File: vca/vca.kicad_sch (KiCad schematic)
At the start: 20 parts, among them U4 STM32F103C6Tx, Y1 Crystal_8Mhz

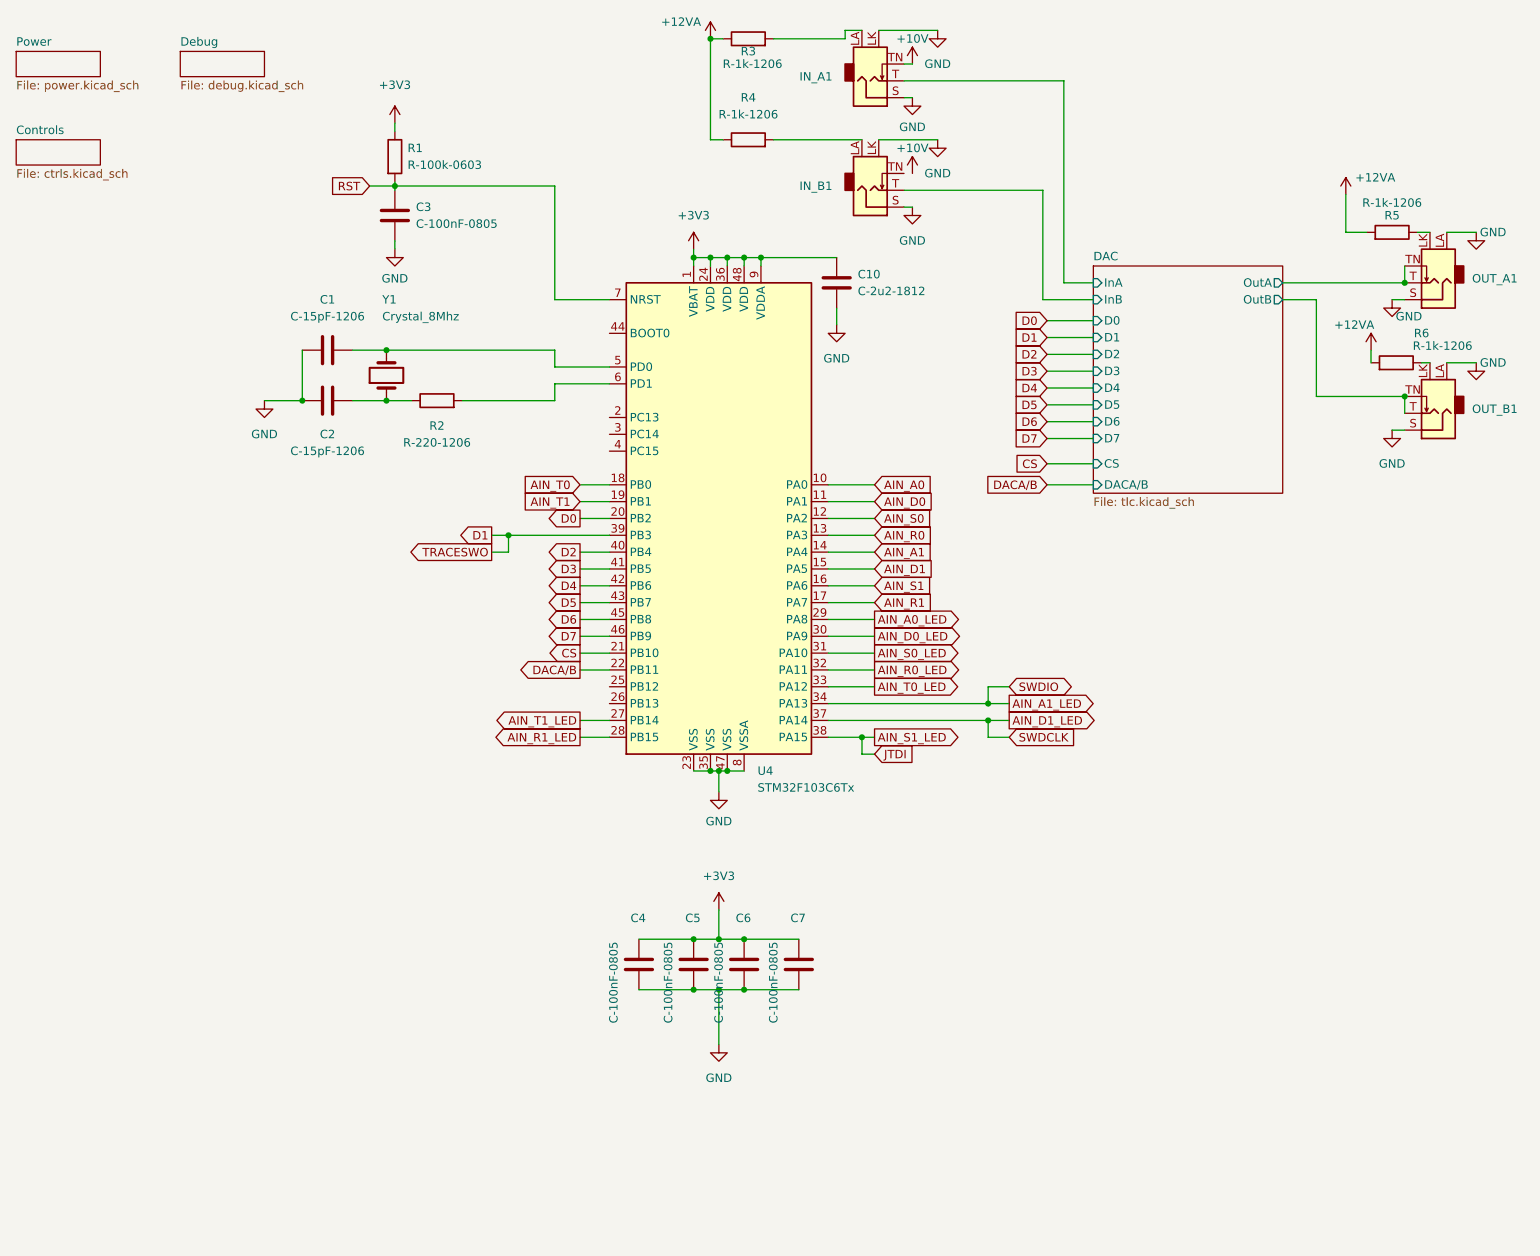
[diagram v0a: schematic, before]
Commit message: working on the PCB
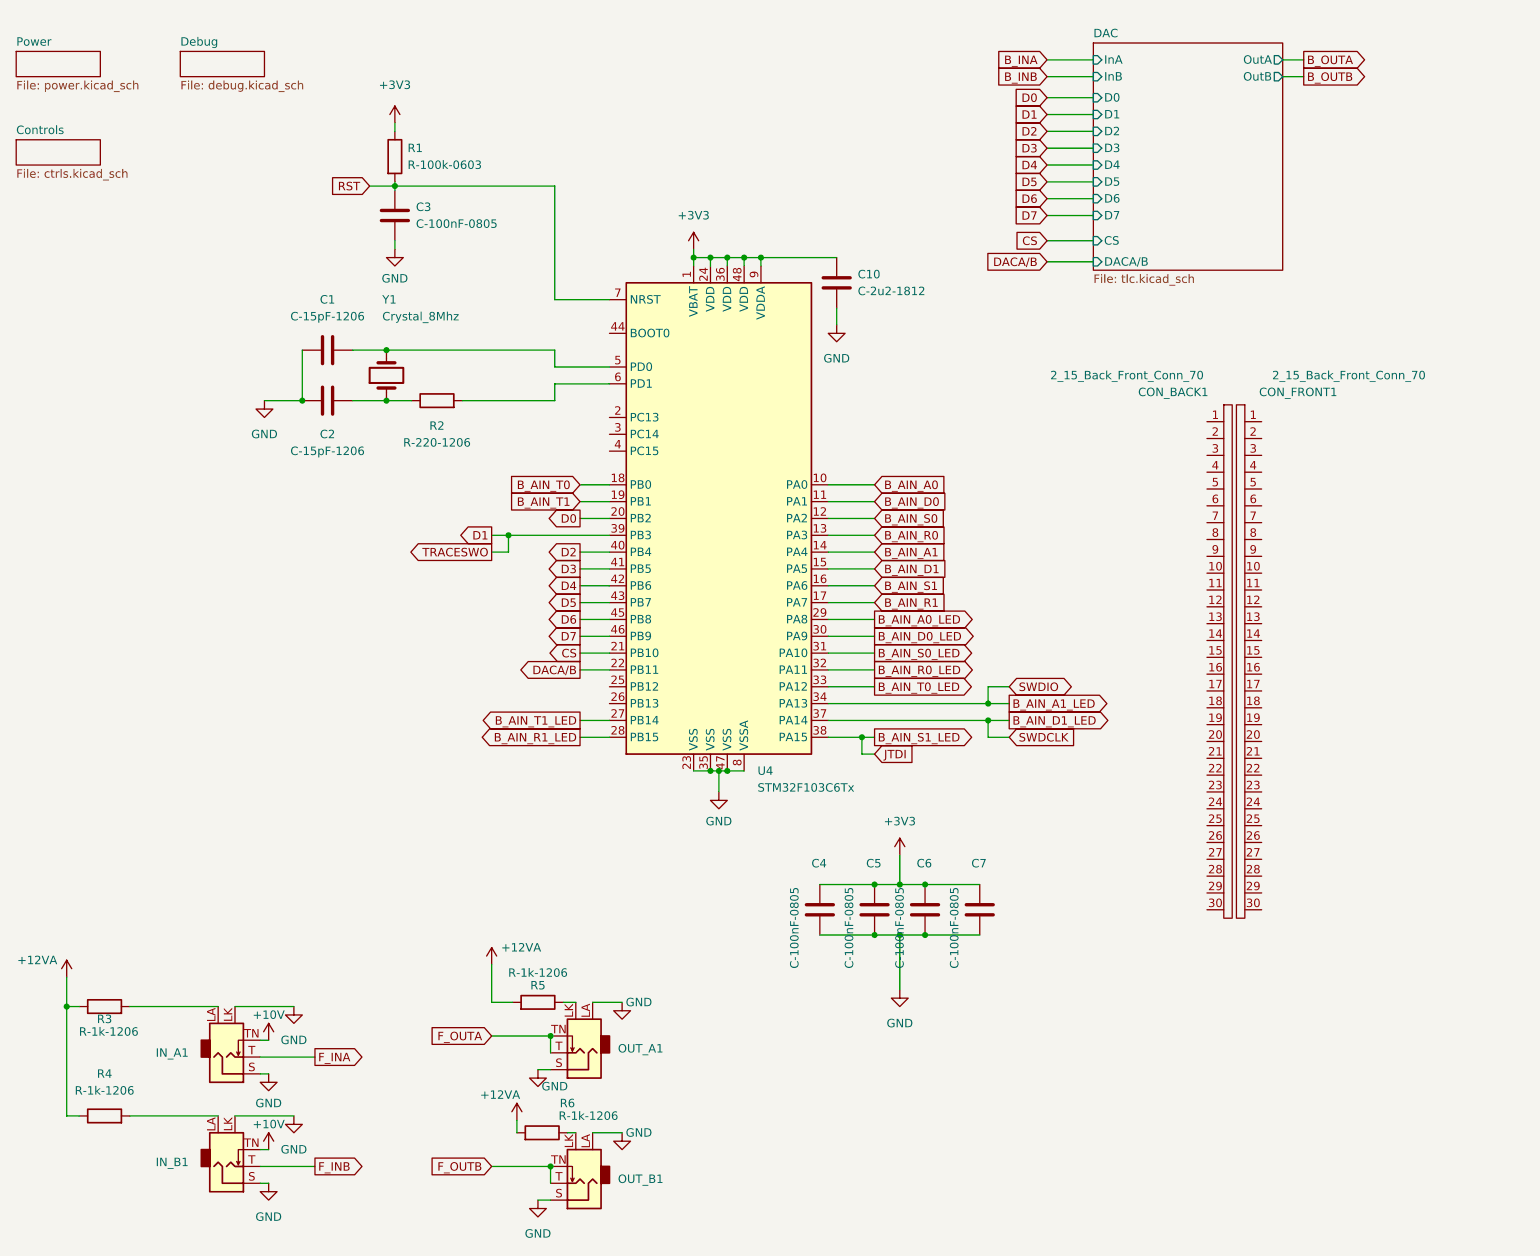
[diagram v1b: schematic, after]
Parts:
- added CON_BACK1, CON_FRONT1: 2_15_Back_Front_Conn_70, eurorack:2_15_back_front_conn_70, symbol eurorack:2_15_Back_Front_Conn_70
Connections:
- net +10V: now also IN_B1.TN
- net AIN_A0 renamed B_AIN_A0
- net AIN_A0_LED renamed B_AIN_A0_LED
- net AIN_A1 renamed B_AIN_A1
- net AIN_A1_LED renamed B_AIN_A1_LED
- net AIN_D0 renamed B_AIN_D0
- net AIN_D0_LED renamed B_AIN_D0_LED
- net AIN_D1 renamed B_AIN_D1
- net AIN_D1_LED renamed B_AIN_D1_LED
- net AIN_R0 renamed B_AIN_R0
- net AIN_R0_LED renamed B_AIN_R0_LED
- net AIN_R1 renamed B_AIN_R1
- net AIN_R1_LED renamed B_AIN_R1_LED
- net AIN_S0 renamed B_AIN_S0
- net AIN_S0_LED renamed B_AIN_S0_LED
- net AIN_S1 renamed B_AIN_S1
- net AIN_S1_LED renamed B_AIN_S1_LED
- net AIN_T0 renamed B_AIN_T0
- net AIN_T0_LED renamed B_AIN_T0_LED
- net AIN_T1 renamed B_AIN_T1
- net AIN_T1_LED renamed B_AIN_T1_LED
- net DAC/InA renamed F_INA
- net DAC/InB renamed F_INB
- net DAC/OutA renamed F_OUTA
- net DAC/OutB renamed F_OUTB
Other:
- moved on the sheet: C4, C5, C6, C7, IN_A1, IN_B1, OUT_A1, OUT_B1, R3, R4, R5, R6

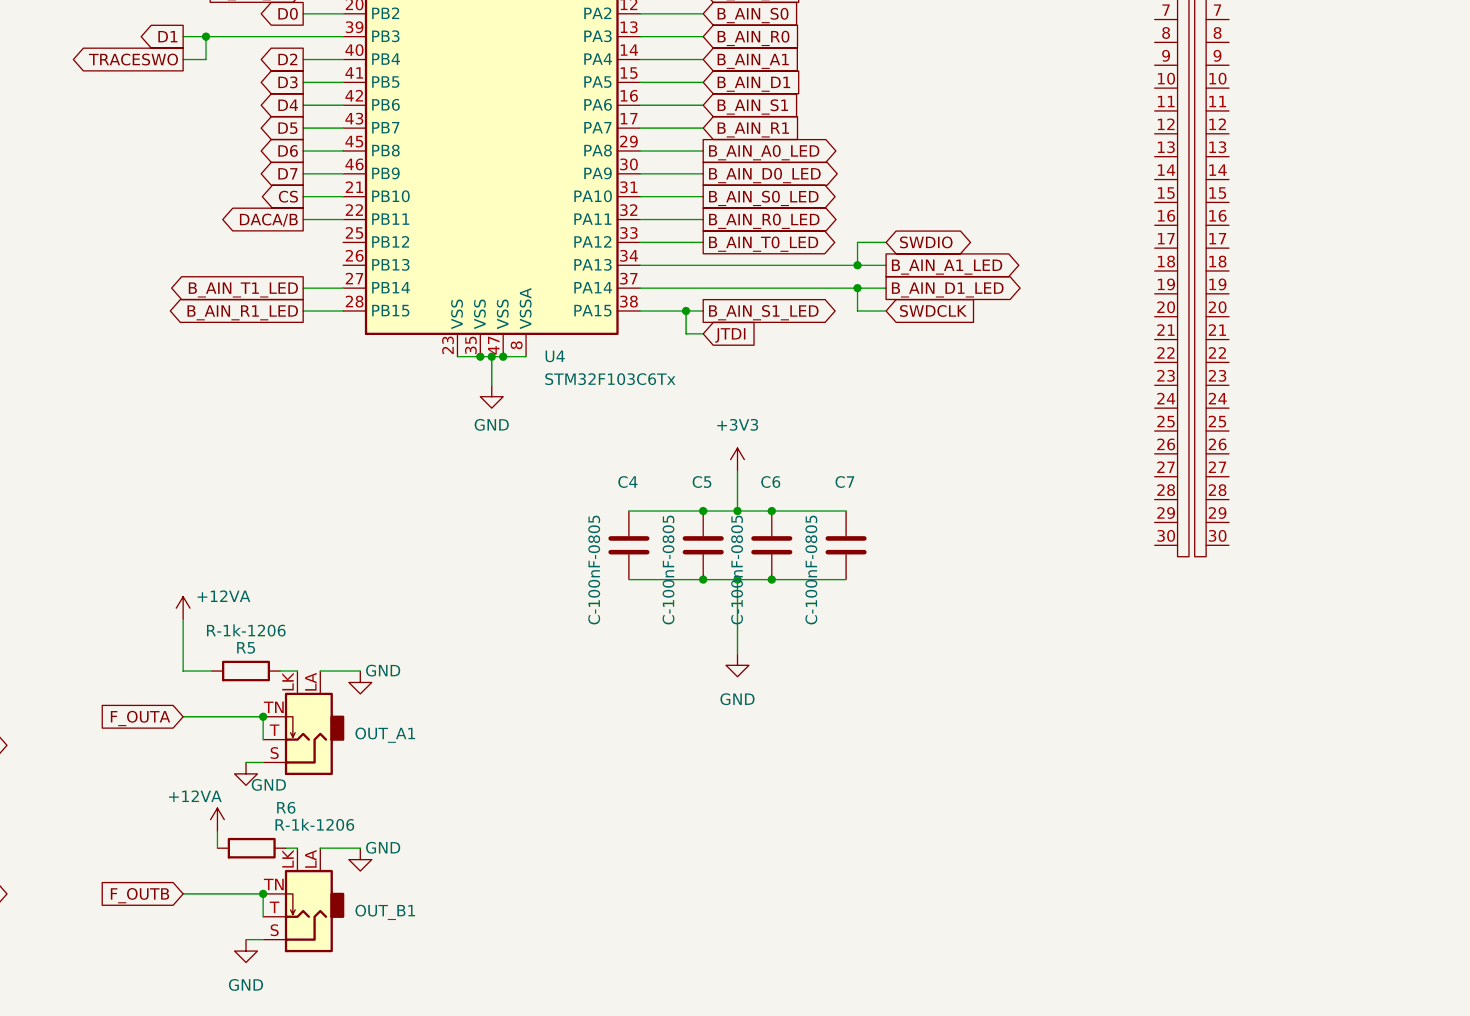
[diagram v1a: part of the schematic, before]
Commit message: working on front panel
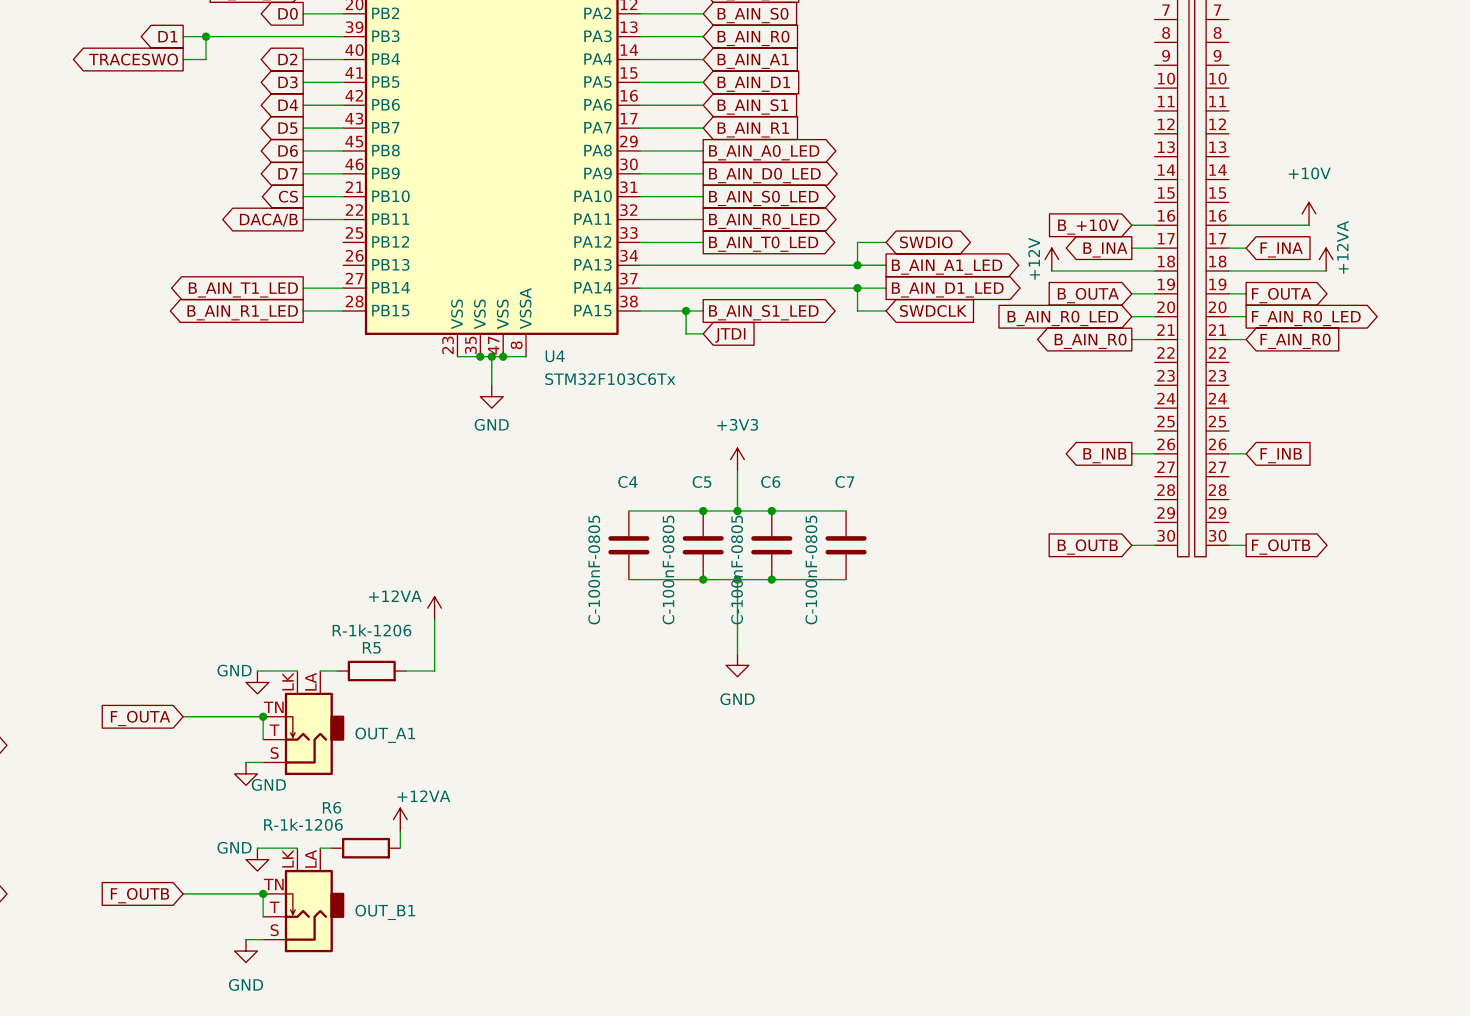
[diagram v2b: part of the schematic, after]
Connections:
- net +10V: now also CON_FRONT1.16
- net +12VA: now also CON_FRONT1.18
- net B_AIN_R0: now also CON_BACK1.21
- net B_AIN_R0_LED: now also CON_BACK1.20
- net B_INA: now also CON_BACK1.17
- net B_INB: now also CON_BACK1.26
- net B_OUTA: now also CON_BACK1.19
- net B_OUTB: now also CON_BACK1.30
- net F_INA: now also CON_FRONT1.17
- net F_INB: now also CON_FRONT1.26
- net F_OUTA: now also CON_FRONT1.19
- net F_OUTB: now also CON_FRONT1.30
- net GND: now also OUT_A1.LK, OUT_B1.LK; no longer OUT_A1.LA, OUT_B1.LA
- net at R6.1: now also OUT_B1.LA; no longer OUT_B1.LK
- net B_+10V: now reaches CON_BACK1.16
- net +12V: now reaches CON_BACK1.18
- net at R5.1: now also OUT_A1.LA; no longer OUT_A1.LK
- net F_AIN_R0_LED: now reaches CON_FRONT1.20
- net F_AIN_R0: now reaches CON_FRONT1.21
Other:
- moved on the sheet: R5, R6

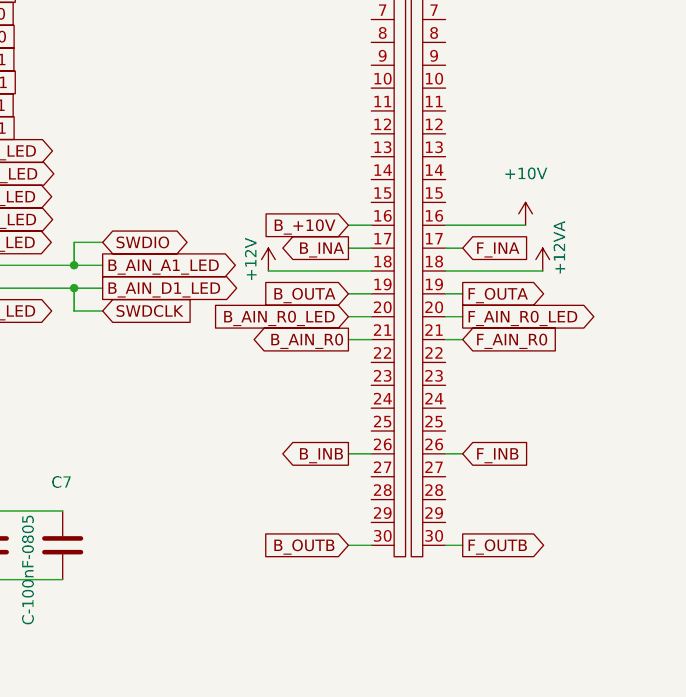
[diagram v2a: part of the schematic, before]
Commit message: working on the front panel
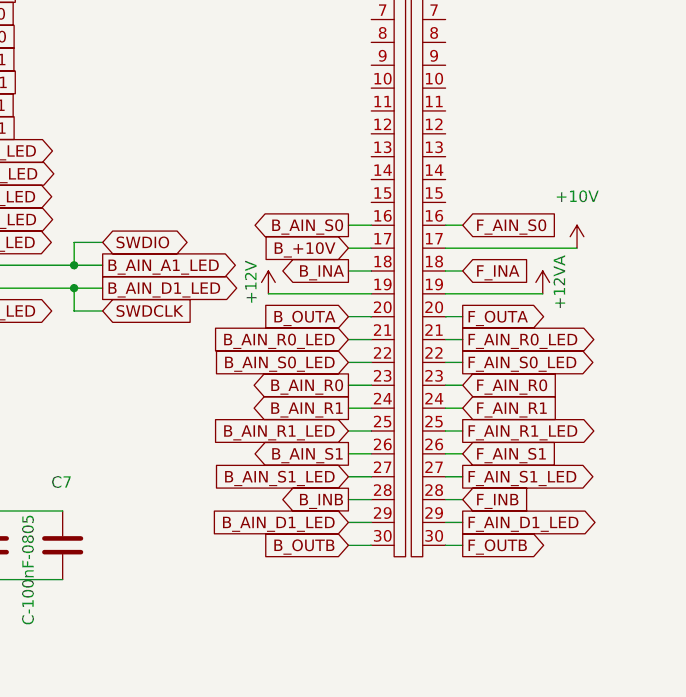
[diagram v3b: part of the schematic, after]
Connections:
- net +10V: now also CON_FRONT1.17; no longer CON_FRONT1.16
- net +12V: now also CON_BACK1.19; no longer CON_BACK1.18
- net +12VA: now also CON_FRONT1.19; no longer CON_FRONT1.18
- net B_+10V: now also CON_BACK1.17; no longer CON_BACK1.16
- net B_AIN_D1_LED: now also CON_BACK1.29
- net B_AIN_R0: now also CON_BACK1.23; no longer CON_BACK1.21
- net B_AIN_R0_LED: now also CON_BACK1.21; no longer CON_BACK1.20
- net B_AIN_R1: now also CON_BACK1.24
- net B_AIN_R1_LED: now also CON_BACK1.25
- net B_AIN_S0: now also CON_BACK1.16
- net B_AIN_S0_LED: now also CON_BACK1.22
- net B_AIN_S1: now also CON_BACK1.26
- net B_AIN_S1_LED: now also CON_BACK1.27
- net B_INA: now also CON_BACK1.18; no longer CON_BACK1.17
- net B_INB: now also CON_BACK1.28; no longer CON_BACK1.26
- net B_OUTA: now also CON_BACK1.20; no longer CON_BACK1.19
- net F_AIN_R0: now also CON_FRONT1.23; no longer CON_FRONT1.21
- net F_AIN_R0_LED: now also CON_FRONT1.21; no longer CON_FRONT1.20
- net F_INA: now also CON_FRONT1.18; no longer CON_FRONT1.17
- net F_INB: now also CON_FRONT1.28; no longer CON_FRONT1.26
- net F_OUTA: now also CON_FRONT1.20; no longer CON_FRONT1.19
- net F_AIN_S0_LED: now reaches CON_FRONT1.22
- net F_AIN_R1: now reaches CON_FRONT1.24
- net F_AIN_R1_LED: now reaches CON_FRONT1.25
- net F_AIN_S1_LED: now reaches CON_FRONT1.27
- net F_AIN_D1_LED: now reaches CON_FRONT1.29
- new net F_AIN_S0: CON_FRONT1.16
- new net F_AIN_S1: CON_FRONT1.26

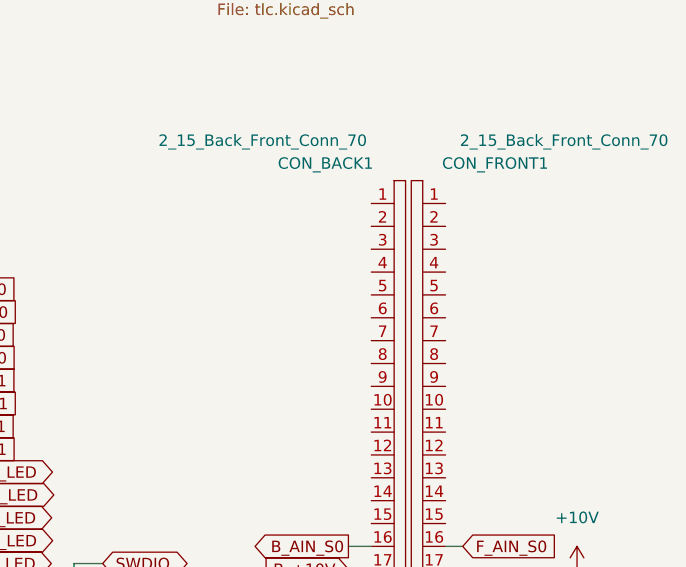
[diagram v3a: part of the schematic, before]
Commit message: working on the front
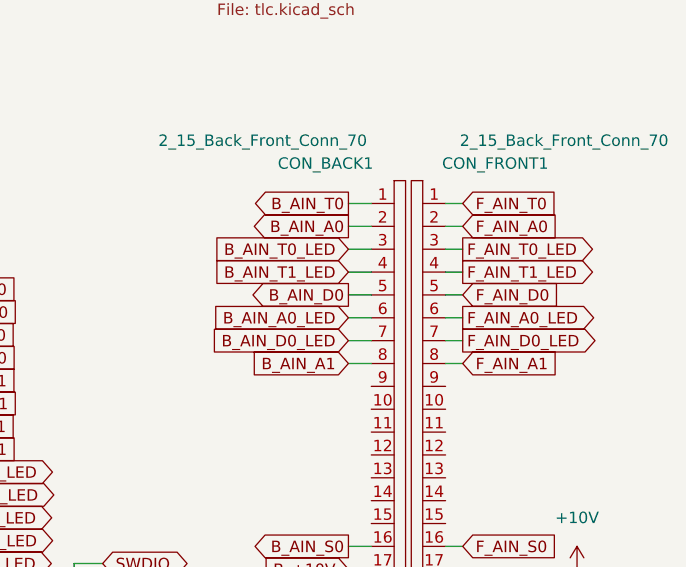
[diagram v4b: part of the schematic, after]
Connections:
- net B_AIN_A0: now also CON_BACK1.2
- net B_AIN_A0_LED: now also CON_BACK1.6
- net B_AIN_A1: now also CON_BACK1.8
- net B_AIN_D0: now also CON_BACK1.5
- net B_AIN_D0_LED: now also CON_BACK1.7
- net B_AIN_T0: now also CON_BACK1.1
- net B_AIN_T0_LED: now also CON_BACK1.3
- net B_AIN_T1_LED: now also CON_BACK1.4
- net F_AIN_T0: now reaches CON_FRONT1.1
- net F_AIN_A0: now reaches CON_FRONT1.2
- net F_AIN_T0_LED: now reaches CON_FRONT1.3
- net F_AIN_T1_LED: now reaches CON_FRONT1.4
- net F_AIN_D0: now reaches CON_FRONT1.5
- net F_AIN_A0_LED: now reaches CON_FRONT1.6
- net F_AIN_D0_LED: now reaches CON_FRONT1.7
- net F_AIN_A1: now reaches CON_FRONT1.8
